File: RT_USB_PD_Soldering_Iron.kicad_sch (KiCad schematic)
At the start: 62 parts, among them J1 USB4105-GF-A, J2 35RASMT4BHNTRX, J3 Conn_02x03_Odd_Even, SW1 SW_Push, SW2 SW_Push, U1 SPX3819M5-L-3-3, U2 BMI270, U3 DRTR5V0U4S-7, U5 STM32G431Kxxx, U6 TPS25982ONRGET, U7 OPA376AIDCKR, U8 STTS22H, Y1 NX2016SA-24MHZ-EXS00A-CS10820

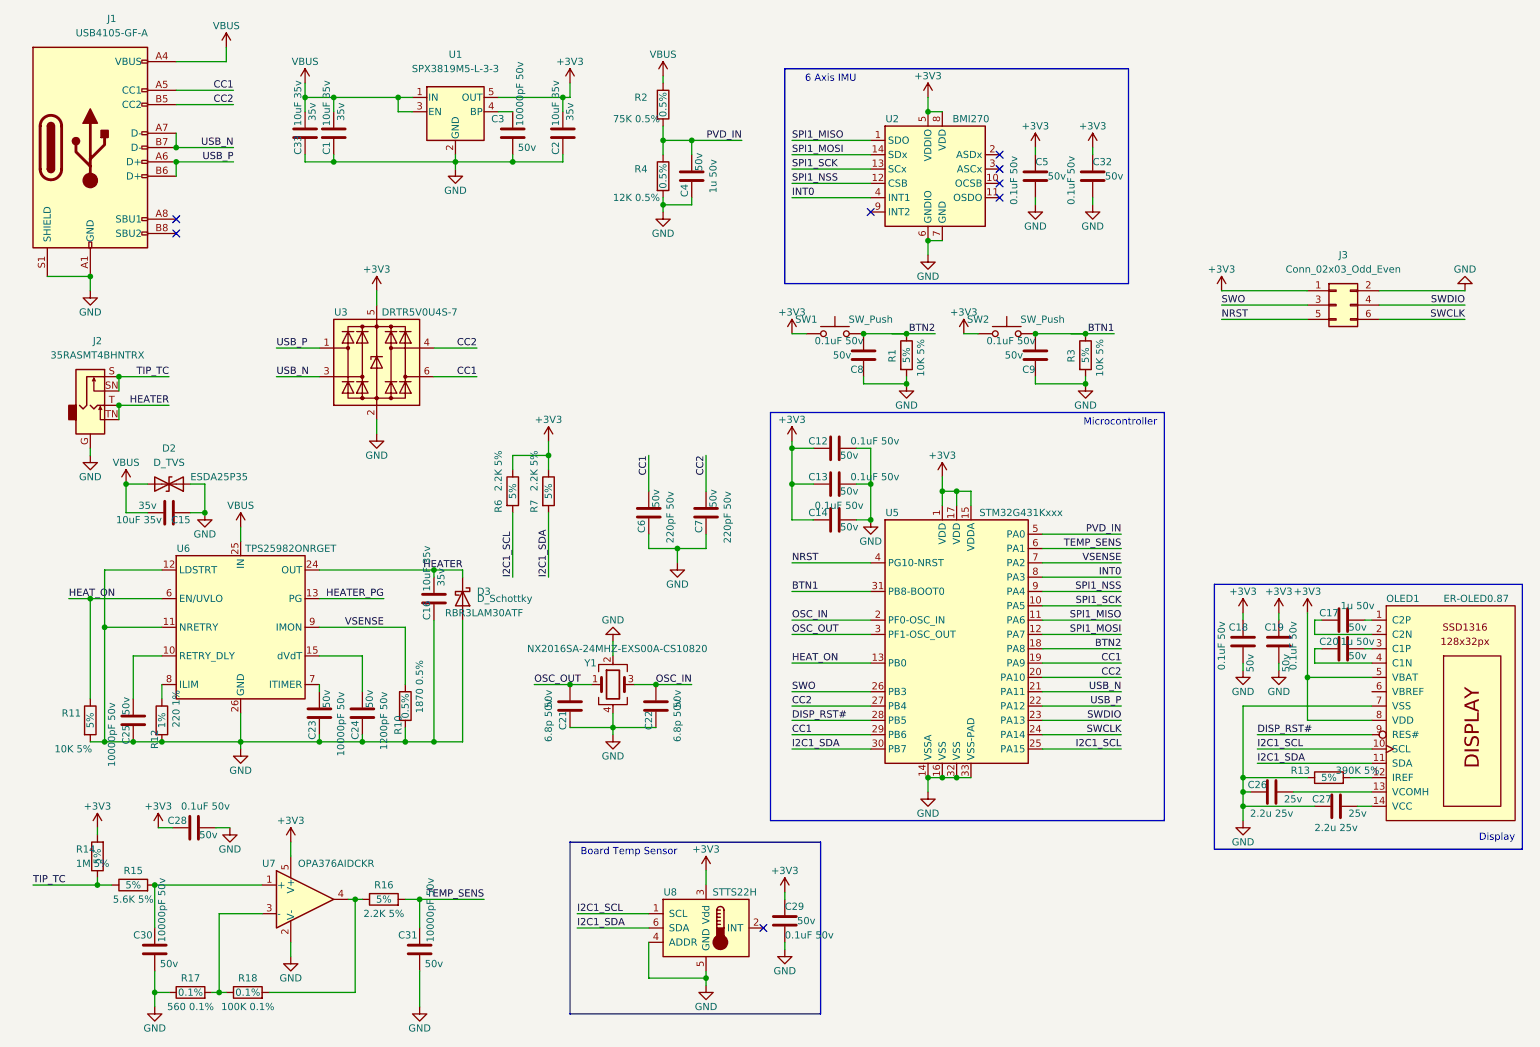
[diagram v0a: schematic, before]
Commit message: First revision 0.1
Rev 0.1 untested unverified.
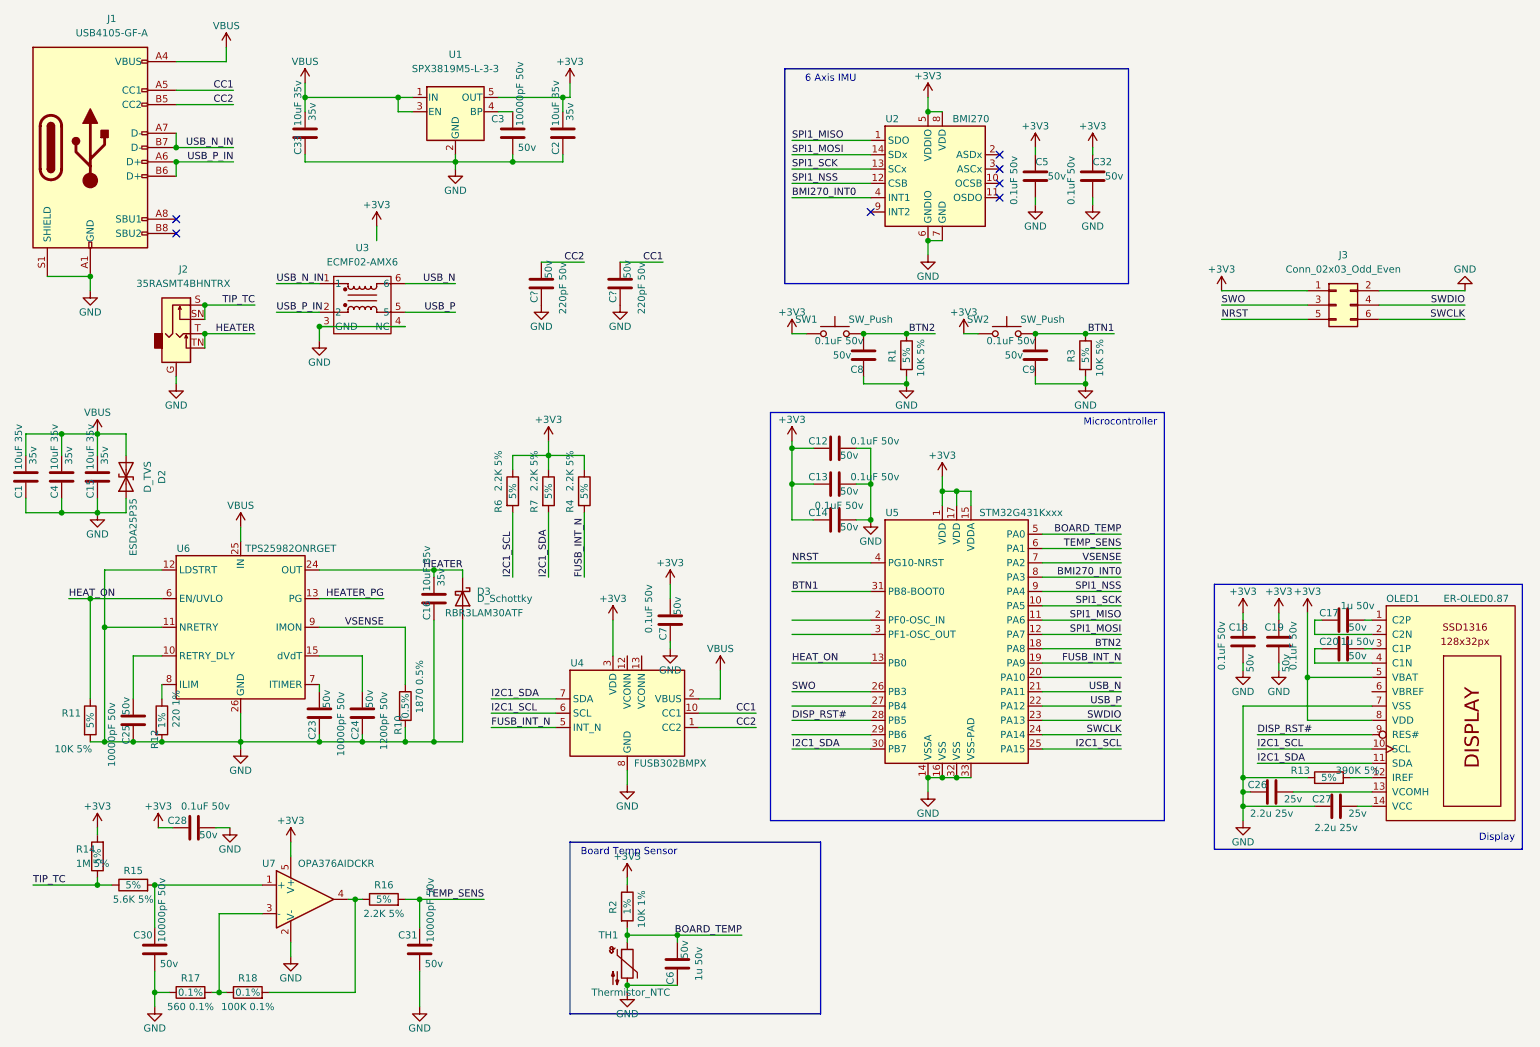
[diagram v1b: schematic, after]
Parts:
- removed C21, C22: 6.8p 50v, Capacitor_SMD:C_0402_1005Metric, symbol Device:C
- removed C29: 0.1uF 50v, Capacitor_SMD:C_0402_1005Metric, symbol Device:C
- removed U3: DRTR5V0U4S-7, Package_TO_SOT_SMD:SOT-363_SC-70-6, symbol Power_Protection:USBLC6-4SC6
- removed U8: STTS22H, Package_DFN_QFN:DFN-6-1EP_2x2mm_P0.65mm_EP1x1.6mm, symbol STTS22HTR:STTS22H
- removed Y1: NX2016SA-24MHZ-EXS00A-CS10820, Crystal:Crystal_SMD_2016-4Pin_2.0x1.6mm, symbol Device:Crystal_GND24
- added C? (x2): 220pF 50v, Capacitor_SMD:C_0402_1005Metric, symbol Device:C
- added TH1: Thermistor_NTC, Resistor_SMD:R_0402_1005Metric, symbol Device:Thermistor_NTC
- added U3: ECMF02-AMX6, Package_DFN_QFN:ST_UQFN-6L_1.5x1.7mm_Pitch0.5mm, symbol ECMF02-AMX6:ECMF02-AMX6
- added U4: FUSB302BMPX, Package_DFN_QFN:WQFN-14-1EP_2.5x2.5mm_P0.5mm_EP1.45x1.45mm, symbol Interface_USB:FUSB302BMPX
- C4: value 1u 50v -> 10uF 35v; footprint Capacitor_SMD:C_0402_1005Metric -> Capacitor_SMD:C_0603_1608Metric_Pad1.05x0.95mm_HandSolder; Voltage 50v -> 35v
- C6: value 220pF 50v -> 1u 50v
- C7: value 220pF 50v -> 0.1uF 50v
- R2: value 75K 0.5% -> 10K 1%; Tolerance 0.5% -> 1%
- R4: value 12K 0.5% -> 2.2K 5%; Tolerance 0.5% -> 5%
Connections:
- net +3V3: now also C7.2, R2.1, R4.1, U4.3 (VDD), U4.4 (VDD)
- net CC1: now also C?.2, U4.10 (CC1), U4.11 (CC1); no longer C6.2, U5.19 (PA9), U5.29 (PB6)
- net CC2: now also C?.2, U4.1 (CC2), U4.14 (CC2); no longer C7.2, U5.20 (PA10), U5.27 (PB4)
- net GND: now also C4.2, C?.1, C?.1, TH1.2, U3.3 (GND), U3.4 (NC), U4.15 (GND), U4.8 (GND), U4.9 (GND); no longer C4.1, R4.2
- net I2C1_SCL: now also U4.6 (SCL)
- net I2C1_SDA: now also U4.7 (SDA)
- net IN: now also C4.1, U4.2 (VBUS); no longer R2.1
- net USB_N: now also U3.6; no longer J1.A7 (D-), J1.B7 (D-)
- net USB_P: now also U3.5; no longer J1.A6 (D+), J1.B6 (D+)
- net INT0 renamed BMI270_INT0
- net OSC_IN: no longer names the net of U5.2 (PF0-OSC_IN)
- net OSC_OUT: no longer names the net of U5.3 (PF1-OSC_OUT)
- net PVD_IN renamed BOARD_TEMP
- net BOARD_TEMP: now also C6.2, TH1.1; no longer C4.2, R4.1
- new net FUSB_INT_N: R4.2, U4.5 (INT_N), U5.19 (PA9)
- new net USB_N_IN: J1.A7 (D-), J1.B7 (D-), U3.1
- new net USB_P_IN: J1.A6 (D+), J1.B6 (D+), U3.2
- no-connect marks 8 -> 7
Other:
- moved on the sheet: C1, C15, D2, J2
